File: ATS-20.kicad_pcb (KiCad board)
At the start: 2 copper layers, 122.1 x 128.5 mm, 81 parts, among them J1 Conn_02x05_Odd_Even, J10 Conn_01x02_Pin, J103 Screw_Terminal_01x02, J13 Conn_01x02_Pin, J15 Conn_01x02_Pin, J17 AudioJack2, J2 AudioJack3, J4 Conn_Coaxial, J6 Screw_Terminal_01x02, J7 Conn_01x04_Pin, J9 Conn_01x02_Pin, Q1 BC847, SW1 SW_Push, SW2 SW_Push, SW3 SW_Push, SW4 SW_Push, SW5 SW_Push, SW6 SW_Push, SW7 SW_SPDT, SW8 RotaryEncoder_Switch, U1 TL072, U2 LM386, U5 TDA1308, U6 L7805, U9 SI4732, Y2 32.768k

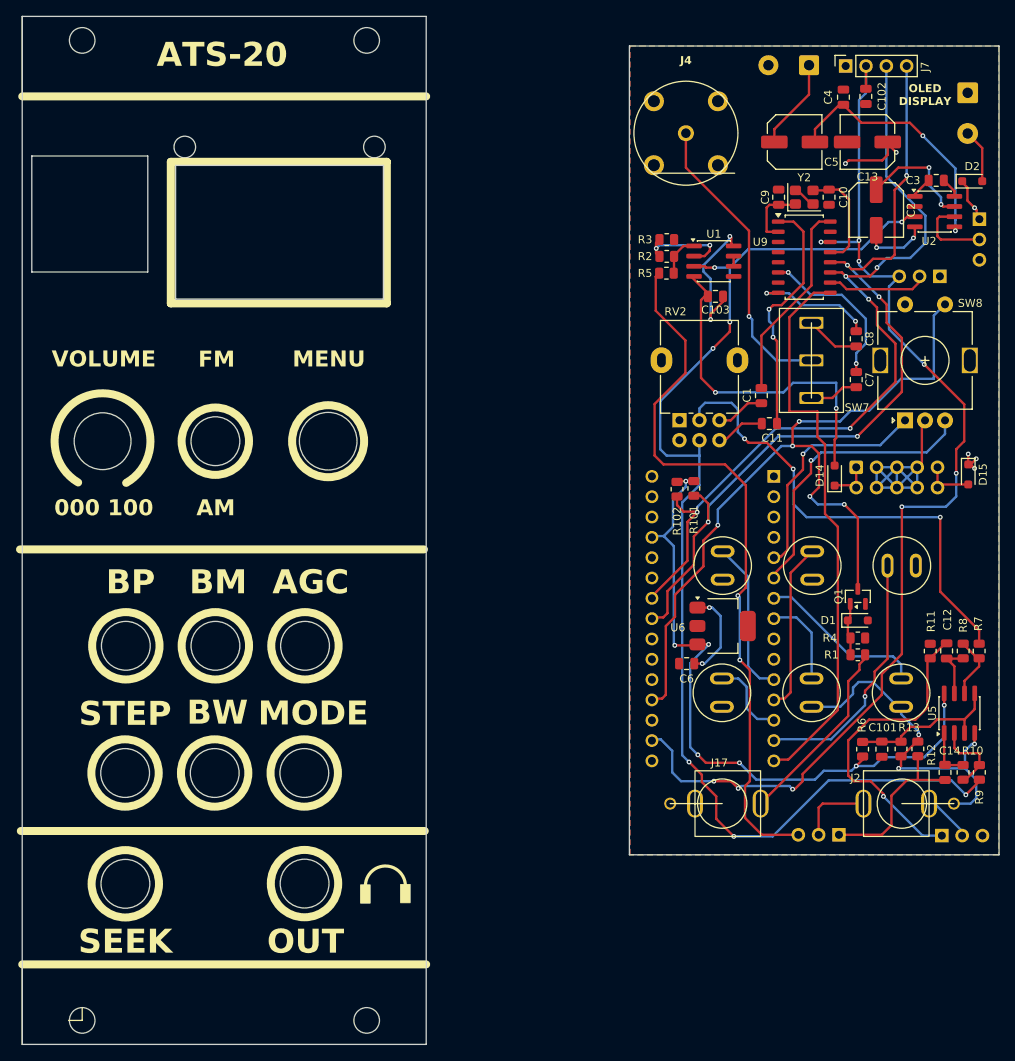
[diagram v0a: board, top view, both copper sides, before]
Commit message: Add files via upload
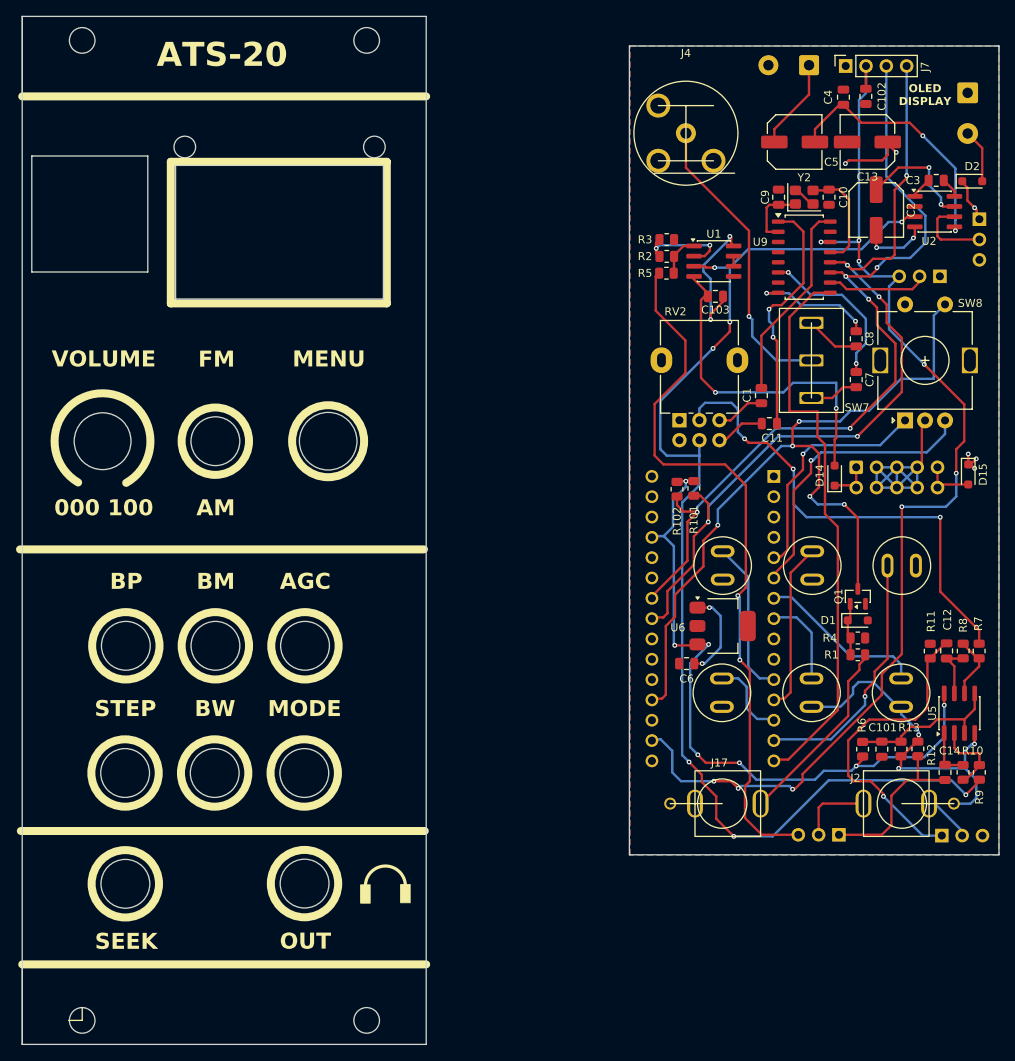
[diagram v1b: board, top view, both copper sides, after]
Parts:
- J4: footprint Library:RS218-4243 -> Library:BNC5-J-P-GN-ST-TH2D
